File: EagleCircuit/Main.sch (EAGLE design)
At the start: 13 parts

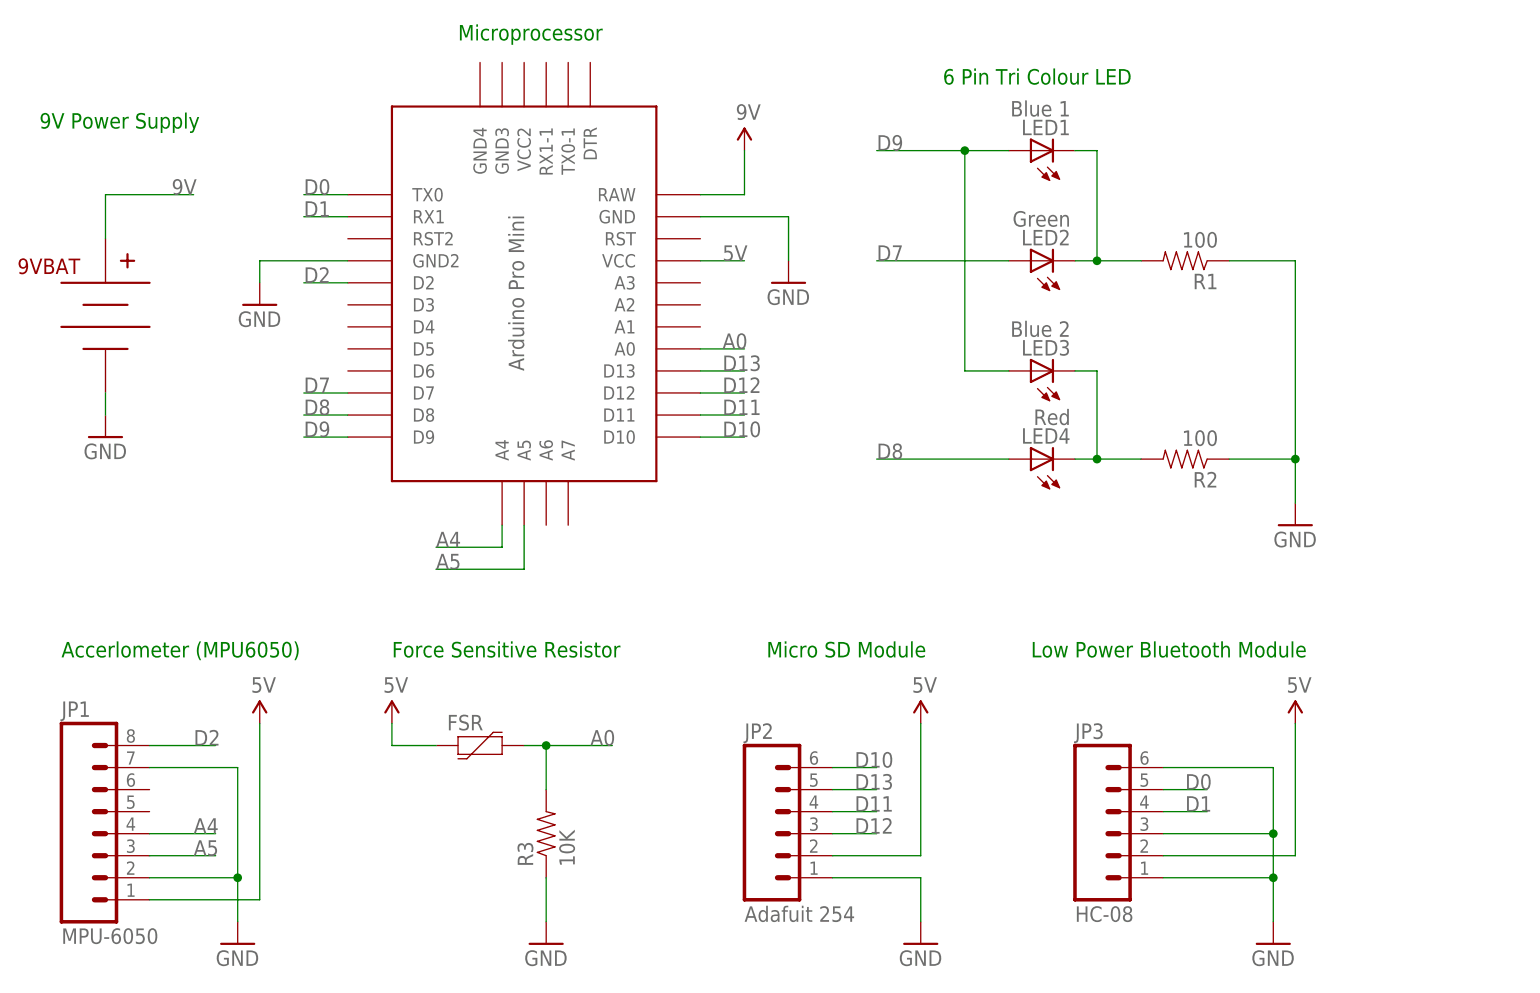
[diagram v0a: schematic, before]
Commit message: Updating Circuit Diagram
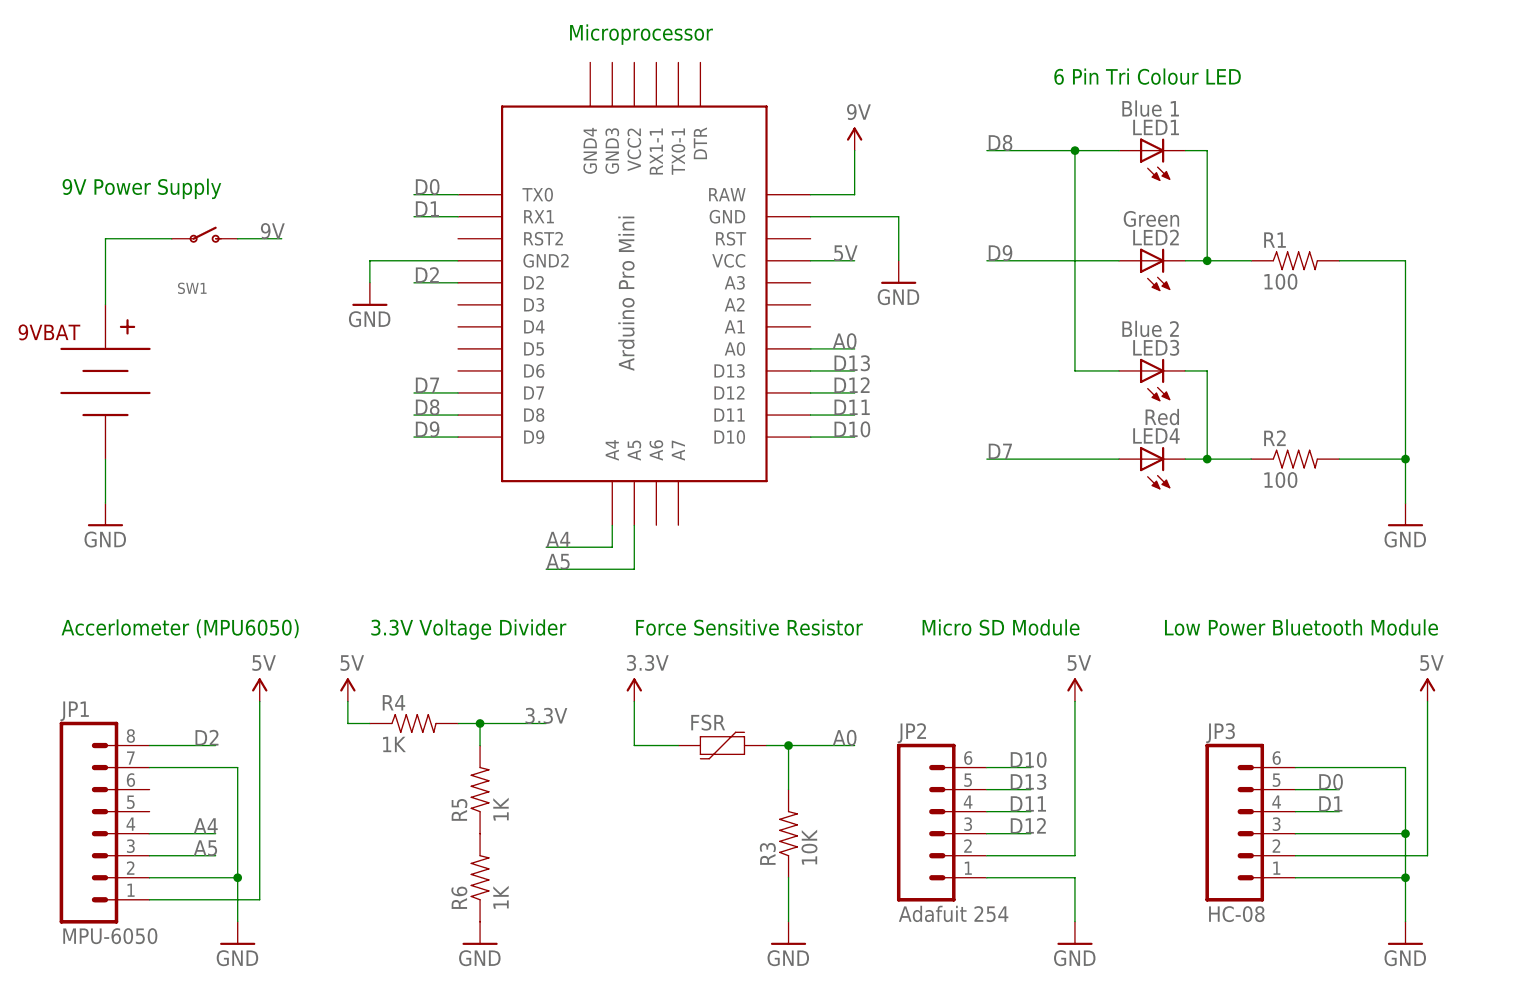
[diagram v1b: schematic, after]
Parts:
- added R4, R5, R6: 1K, SparkFun-Passives:RESISTORAXIAL-0.3
- added SW1: (no value), microbuilder:SWITCH_SPST
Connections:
- new net 3.3V: FSR.1, R4.2, R5.2
- new net N$1: R5.1, R6.2
- new net POWERSWITCH: 9VBAT.V+, SW1.P
- net 5V: now also R4.1; no longer FSR.1
- net 9V: now also SW1.S; no longer 9VBAT.V+
- net BG_LED: now also R1.1; no longer R1.2
- net D7: now also LED4.A; no longer LED2.A
- net D8: now also LED1.A, LED3.A; no longer LED4.A
- net D9: now also LED2.A; no longer LED1.A, LED3.A
- net GND: now also R1.2, R2.2, R6.1; no longer R1.1, R2.1
- net RB_LED: now also R2.1; no longer R2.2
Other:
- note added: "3.3V Voltage Divider"
- moved on the sheet: 9VBAT, FSR, JP2, JP3, LED1, LED2, LED3, LED4, R1, R2, R3
